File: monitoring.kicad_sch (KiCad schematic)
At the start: 146 parts, among them Q42 NMOS, Q43 PMOS, Q44 NMOS, Q45 PMOS, Q46 PMOS, Q47 NMOS, Q48 NMOS, Q49 PMOS, Q50 NMOS, Q51 NMOS, Q52 PMOS, Q53 NMOS, Q60 NMOS, Q61 NMOS, SW1 SW_Push, U1 BQ76940DBT, U2 BQ76940DBT, U3 ISO1541

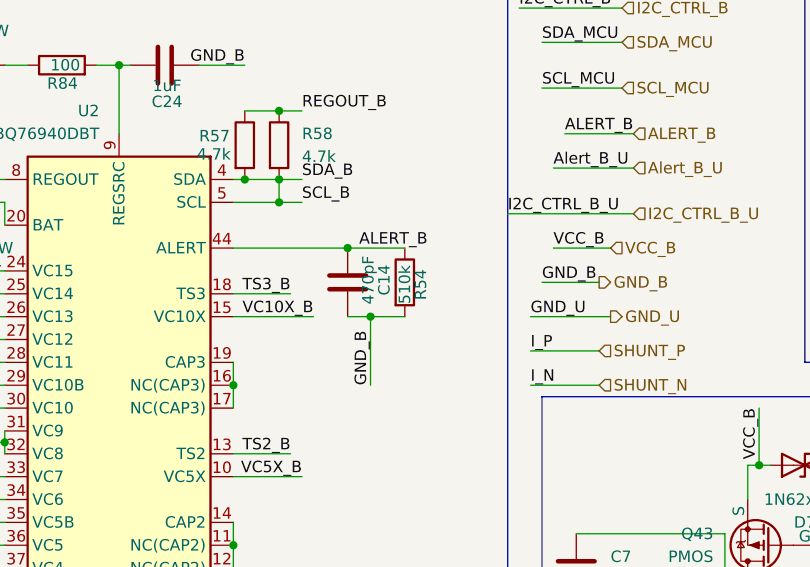
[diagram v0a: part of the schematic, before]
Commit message: MVP Friday
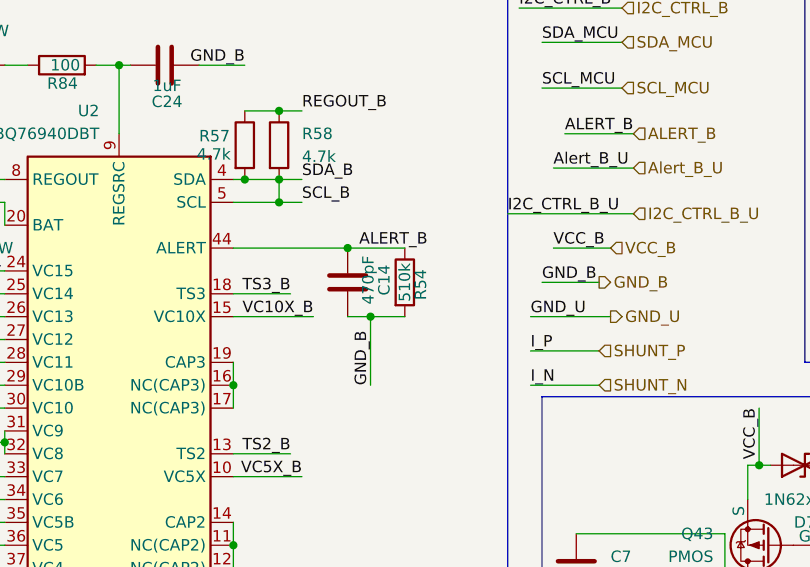
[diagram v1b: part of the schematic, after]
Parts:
- C20, C21: footprint (none) -> Capacitor_SMD:C_1206_3216Metric; LCSC (none) -> C5189849
- R44, R45, R55, R56, R57, R58, R86, R87: footprint (none) -> Resistor_SMD:R_0603_1608Metric; LCSC (none) -> C2077906
- R46: footprint (none) -> Resistor_SMD:R_0603_1608Metric; LCSC (none) -> C103548
- R47: footprint (none) -> Resistor_SMD:R_0603_1608Metric; LCSC (none) -> C2930043
- R48, R50: footprint (none) -> Resistor_SMD:R_0402_1005Metric; LCSC (none) -> C325551
- R49, R51, R52, R53, R59, R62, R72: footprint (none) -> Resistor_SMD:R_0603_1608Metric; LCSC (none) -> C23156
- R54, R61: footprint (none) -> Resistor_SMD:R_0603_1608Metric; LCSC (none) -> C2907178
